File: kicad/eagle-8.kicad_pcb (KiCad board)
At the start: 4 copper layers, 127.1 x 96.7 mm, 46 parts, among them J1 SC242, J2 PGA387

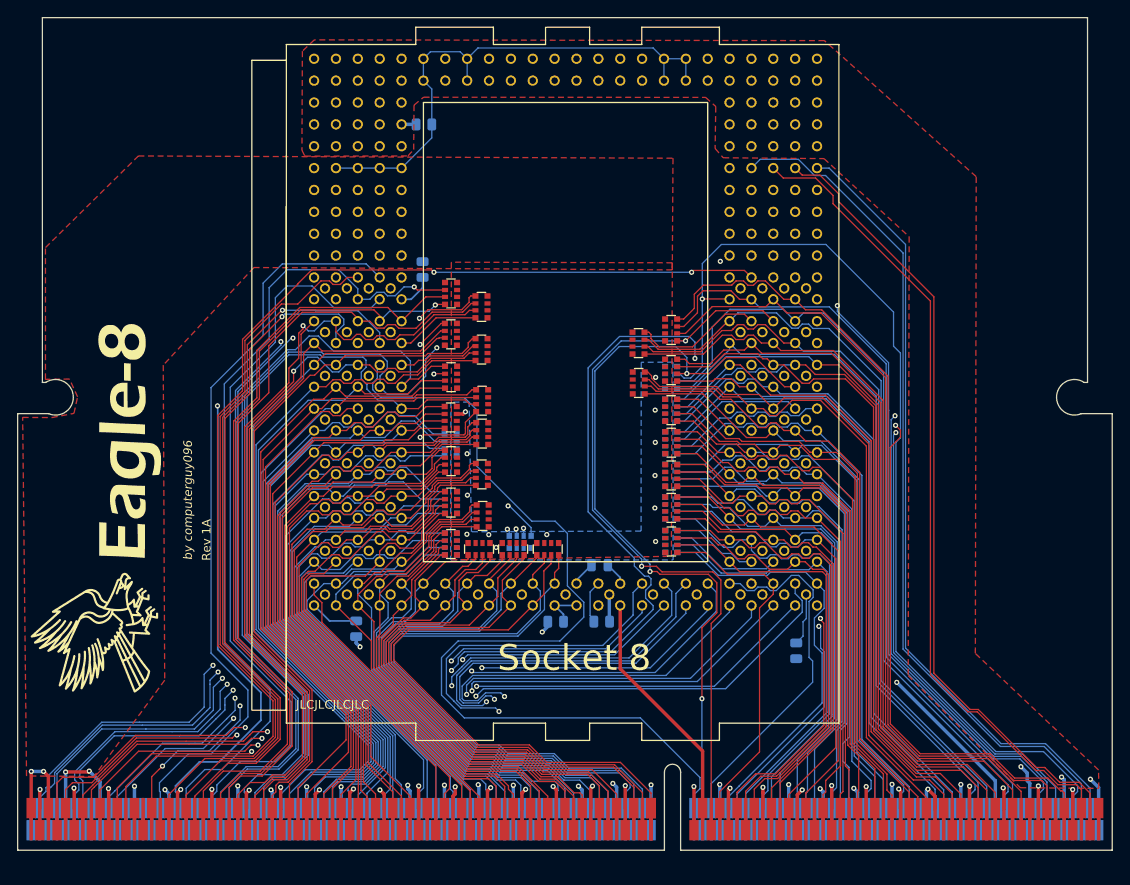
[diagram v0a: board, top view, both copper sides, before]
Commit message: more improvements
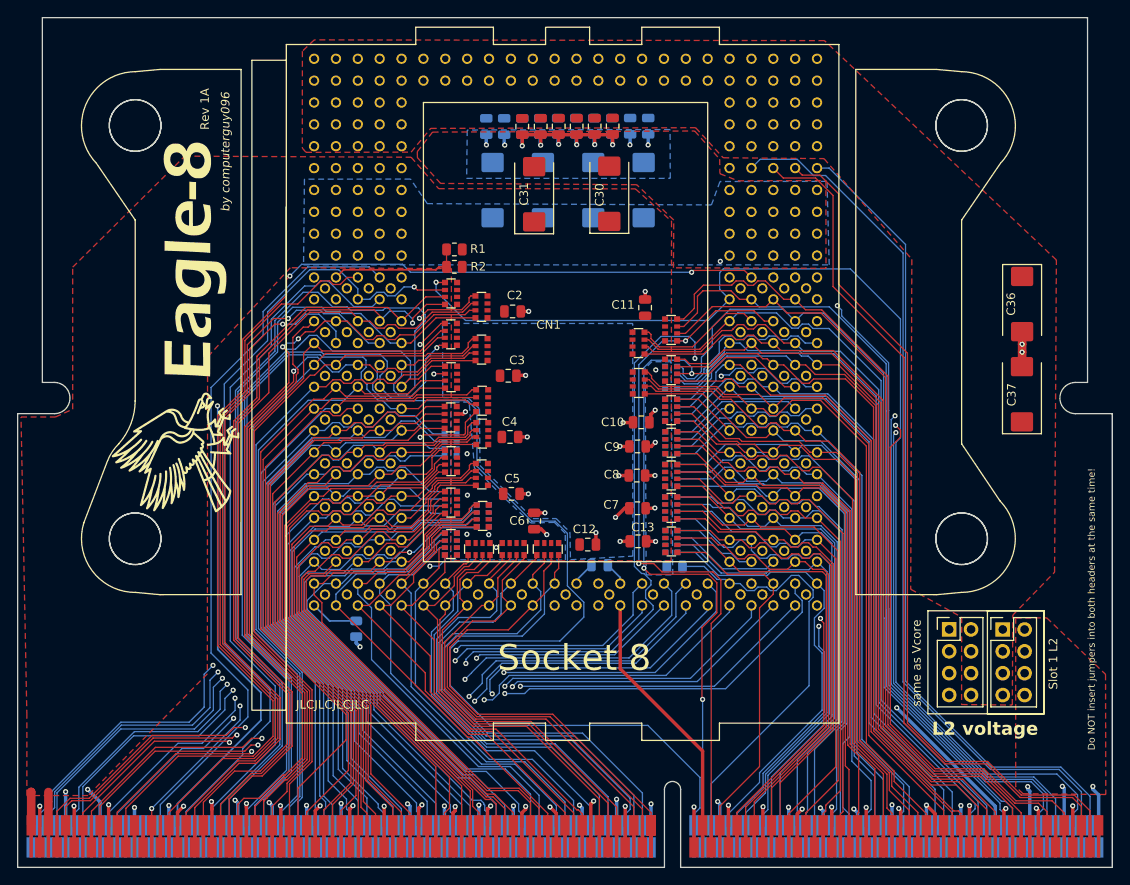
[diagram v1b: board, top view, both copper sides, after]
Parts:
- removed R4: 0, Resistor_SMD:R_0805_2012Metric
- removed R7, R8: 1K, Resistor_SMD:R_0805_2012Metric
- added C10: 100n, Capacitor_SMD:C_0805_2012Metric, F.Cu at (164.0, 82.2)
- added C11: 100n, Capacitor_SMD:C_0805_2012Metric, F.Cu at (164.5, 68.9)
- added C12: 100n, Capacitor_SMD:C_0805_2012Metric, F.Cu at (157.8, 96.4)
- added C13: 100n, Capacitor_SMD:C_0805_2012Metric, F.Cu at (163.7, 96.0)
- added C14: 100n, Capacitor_SMD:C_0805_2012Metric, B.Cu at (158.6, 47.8)
- added C15: 100n, Capacitor_SMD:C_0805_2012Metric, B.Cu at (154.4, 47.8)
- added C16: 100n, Capacitor_SMD:C_0805_2012Metric, B.Cu at (150.2, 47.9)
- added C17: 100n, Capacitor_SMD:C_0805_2012Metric, B.Cu at (152.3, 47.9)
- added C18: 100n, Capacitor_SMD:C_0805_2012Metric, B.Cu at (160.7, 47.8)
- added C19: 100n, Capacitor_SMD:C_0805_2012Metric, B.Cu at (146.0, 47.9)
- added C2: 100n, Capacitor_SMD:C_0805_2012Metric, F.Cu at (149.1, 69.3)
- added C20: 100n, Capacitor_SMD:C_0805_2012Metric, B.Cu at (156.5, 47.8)
- added C21: 100n, Capacitor_SMD:C_0805_2012Metric, B.Cu at (148.1, 47.9)
- added C22: 100n, Capacitor_SMD:C_0805_2012Metric, B.Cu at (162.8, 47.8)
- added C23: 100n, Capacitor_SMD:C_0805_2012Metric, B.Cu at (164.8, 47.8)
- added C24: 100n, Capacitor_SMD:C_0805_2012Metric, F.Cu at (152.4, 47.9)
- added C25: 100n, Capacitor_SMD:C_0805_2012Metric, F.Cu at (158.6, 47.8)
- added C26: 100n, Capacitor_SMD:C_0805_2012Metric, F.Cu at (160.7, 47.8)
- added C27: 100n, Capacitor_SMD:C_0805_2012Metric, F.Cu at (150.2, 47.9)
- added C28: 100n, Capacitor_SMD:C_0805_2012Metric, F.Cu at (154.4, 47.8)
- added C29: 100n, Capacitor_SMD:C_0805_2012Metric, F.Cu at (156.5, 47.8)
- added C3: 100n, Capacitor_SMD:C_0805_2012Metric, F.Cu at (148.6, 76.8)
- added C30: 47uF, Capacitor_Tantalum_SMD:CP_EIA-7343-40_Kemet-Y_HandSolder, F.Cu at (160.3, 55.7)
- added C31: 47uF, Capacitor_Tantalum_SMD:CP_EIA-7343-40_Kemet-Y_HandSolder, F.Cu at (151.6, 55.7)
- added C32: 47uF, Capacitor_Tantalum_SMD:CP_EIA-7343-40_Kemet-Y_HandSolder, B.Cu at (146.8, 55.2)
- added C33: 47uF, Capacitor_Tantalum_SMD:CP_EIA-7343-40_Kemet-Y_HandSolder, B.Cu at (152.6, 55.2)
- added C34: 47uF, Capacitor_Tantalum_SMD:CP_EIA-7343-40_Kemet-Y_HandSolder, B.Cu at (158.5, 55.2)
- added C35: 47uF, Capacitor_Tantalum_SMD:CP_EIA-7343-40_Kemet-Y_HandSolder, B.Cu at (164.3, 55.2)
- added C36: 47uF, Capacitor_Tantalum_SMD:CP_EIA-7343-40_Kemet-Y_HandSolder, F.Cu at (208.3, 68.5)
- added C37: 47uF, Capacitor_Tantalum_SMD:CP_EIA-7343-40_Kemet-Y_HandSolder, F.Cu at (208.3, 79.0)
- added C4: 100n, Capacitor_SMD:C_0805_2012Metric, F.Cu at (148.8, 83.9)
- added C5: 100n, Capacitor_SMD:C_0805_2012Metric, F.Cu at (149.0, 90.5)
- added C6: 100n, Capacitor_SMD:C_0805_2012Metric, F.Cu at (151.6, 93.7)
- added C7: 100n, Capacitor_SMD:C_0805_2012Metric, F.Cu at (163.6, 92.2)
- added C8: 100n, Capacitor_SMD:C_0805_2012Metric, F.Cu at (163.5, 88.4)
- added C9: 100n, Capacitor_SMD:C_0805_2012Metric, F.Cu at (163.6, 85.0)
- added CN1: AM3 bracket, eagle-8:AM3 bracket, F.Cu at (153.3, 71.7)
- added H1: 6mm, MountingHole:MountingHole_6mm, F.Cu at (201.2, 47.7)
- added H2: 6mm, MountingHole:MountingHole_6mm, F.Cu at (201.2, 95.7)
- added H3: 6mm, MountingHole:MountingHole_6mm, F.Cu at (105.2, 47.7)
- added H4: 6mm, MountingHole:MountingHole_6mm, F.Cu at (105.2, 95.7)
- added J3: same as Vcore, Connector_PinHeader_2.54mm:PinHeader_2x04_P2.54mm_Vertical, F.Cu at (199.8, 106.3)
- added J4: Slot 1 L2, Connector_PinHeader_2.54mm:PinHeader_2x04_P2.54mm_Vertical, F.Cu at (206.0, 106.3)
- added R14: 56R, Resistor_SMD:R_0805_2012Metric, B.Cu at (167.9, 99.0)
- R1, R2: value 1K -> 150R; moved to F.Cu
- R3: value 150R? -> 150R
- moved R2 42.9 mm to (142.3, 64.2)
- moved REF** 23.0 mm to (110.7, 85.4)
- moved G*** 22.4 mm to (112.2, 63.4)
- moved RN16 5.31 mm to (145.6, 93.1), turned to 180 degrees
- moved R1 4.37 mm to (142.3, 62.1), turned to 180 degrees
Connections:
- J2 pad A23: Net-(J2D-TESTHI-PadA23) -> Vcore
- J2 pad A25: Net-(J2D-TESTHI-PadA23) -> Vcore
- J2 pad AA1: unconnected-(J2C-BR2#-PadAA1) -> /BR2
- J2 pad AE39: Net-(J2D-TESTHI-PadAE39) -> Vcore
- J2 pad AS39: Net-(J2D-TESTLO-PadAS39) -> GND
- J2 pad AS41: Net-(J2D-TESTLO-PadAS39) -> GND
- J2 pad AS43: Net-(J2D-TESTLO-PadAS39) -> GND
- J2 pad AS45: Net-(J2D-TESTLO-PadAS39) -> GND
- J2 pad AU1: VccL2 -> VccS
- J2 pad AU39: VccL2 -> VccS
- J2 pad AU43: VccL2 -> VccS
- J2 pad AU47: VccL2 -> VccS
- J2 pad AU5: VccL2 -> VccS
- J2 pad AU9: VccL2 -> VccS
- J2 pad AW3: VccL2 -> VccS
- J2 pad AW41: VccL2 -> VccS
- J2 pad AW45: VccL2 -> VccS
- J2 pad AW7: VccL2 -> VccS
- J2 pad AY1: VccL2 -> VccS
- J2 pad AY3: VccL2 -> VccS
- J2 pad AY39: VccL2 -> VccS
- J2 pad AY41: VccL2 -> VccS
- J2 pad AY43: VccL2 -> VccS
- J2 pad AY45: VccL2 -> VccS
- J2 pad AY47: VccL2 -> VccS
- J2 pad AY5: VccL2 -> VccS
- J2 pad AY7: VccL2 -> VccS
- J2 pad AY9: VccL2 -> VccS
- J2 pad B2: Net-(J2C-CPUPRES#) -> unconnected-(J2C-CPUPRES#-PadB2)
- J2 pad BA13: Net-(J2D-TESTLO-PadAS39) -> GND
- J2 pad BA15: Net-(J2D-TESTLO-PadAS39) -> GND
- J2 pad BA3: VccL2 -> VccS
- J2 pad BA33: Net-(J2D-TESTLO-PadAS39) -> GND
- J2 pad BA37: Net-(J2D-TESTLO-PadAS39) -> GND
- J2 pad BA41: VccL2 -> VccS
- J2 pad BA45: VccL2 -> VccS
- J2 pad BA7: VccL2 -> VccS
- J2 pad BC13: Net-(J2D-TESTLO-PadAS39) -> GND
- J2 pad BC15: Net-(J2D-TESTLO-PadAS39) -> GND
- J2 pad BC19: VccL2 -> VccS
- J2 pad BC23: VccL2 -> VccS
- J2 pad BC27: VccL2 -> VccS
- J2 pad BC31: VccL2 -> VccS
- J2 pad BC33: Net-(J2D-TESTLO-PadAS39) -> GND
- J2 pad BC37: Net-(J2D-TESTLO-PadAS39) -> GND
- J2 pad C21: Net-(J2D-TESTLO-PadC21) -> GND
- J2 pad U9: unconnected-(J2C-BR3#-PadU9) -> /BR3
- R1 pad 1: Vcore -> VTT
- R1 pad 2: Net-(J2D-TESTHI-PadAE39) -> Net-(J2D-VREF0)
- R2 pad 1: Net-(J2D-TESTHI-PadA23) -> VTT
- R2 pad 2: Vcore -> Net-(J2D-VREF0)
- RN10 pad 1: /D15 -> /D12
- RN10 pad 2: /D12 -> /D14
- RN11 pad 1: /D11 -> /D17
- RN11 pad 2: /D17 -> /D11
- RN11 pad 3: /D10 -> /D15
- RN11 pad 4: /D14 -> /D10
- RN12 pad 4: /D23 -> /D25
- RN13 pad 1: /D18 -> /D22
- RN13 pad 2: /D22 -> /D21
- RN13 pad 3: /D13 -> /D18
- RN13 pad 4: /D20 -> /D13
- RN14 pad 1: /D16 -> /D24
- RN14 pad 2: /D19 -> /D20
- RN14 pad 3: /D26 -> /D16
- RN14 pad 4: /D29 -> /D19
- RN16 pad 5: /D21 -> /D23
- RN16 pad 6: /D24 -> /D26
- RN16 pad 7: /D25 -> /D29
- RN16 pad 8: /D38 -> /D31
- RN17 pad 5: /D31 -> /D38
- RN27 pad 5: /REQ3 -> /REQ2
- RN27 pad 7: /REQ2 -> /REQ4
- RN27 pad 8: /REQ4 -> /REQ0
- RN28 pad 5: unconnected-(RN28-R4.2-Pad5) -> /AERR
- RN30 pad 5: unconnected-(RN30-R4.2-Pad5) -> /HIT
- RN30 pad 6: /AERR -> /BR2
- RN30 pad 7: /HIT -> /LOCK
- RN30 pad 8: /LOCK -> /REQ3
- RN35 pad 5: /REQ0 -> /RSP
- RN35 pad 6: /RSP -> /BR3
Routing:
- net Net-(J2D-TESTLO-PadAS39): track 62.0 -> 0.00 mm
- net GND: track 81.9 -> 123.6 mm, vias 30 -> 54
- net /AERR: track 115.6 -> 138.5 mm
- net /BR2: track 0.00 -> 21.2 mm
- net /PRDY: track 89.8 -> 110.6 mm, vias 1 -> 0
- net /D1: track 64.6 -> 53.8 mm
- net /IGNNE: track 102.1 -> 91.5 mm
- net /D5: track 59.8 -> 49.2 mm
- net /D3: track 62.5 -> 51.9 mm
- net /D38: track 70.9 -> 60.7 mm, vias 1 -> 0
- net /D24: track 67.9 -> 58.0 mm
- net /FERR: track 97.8 -> 88.3 mm
- net /D8: track 56.8 -> 47.4 mm
- net /TDI: track 95.4 -> 86.0 mm
- net /D25: track 68.4 -> 59.4 mm, vias 1 -> 0
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- added copper zone on B.Cu, net GND
- added copper zone on F.Cu, net GND
- added copper zone on F.Cu, net VccS
- added copper zone on B.Cu, net Vcore
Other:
- board size 127.1 x 96.7 mm -> 127.1 x 98.7 mm
- board text added: "Do NOT insert jumpers into both headers at the same time!"
- board text added: "L2 voltage"
